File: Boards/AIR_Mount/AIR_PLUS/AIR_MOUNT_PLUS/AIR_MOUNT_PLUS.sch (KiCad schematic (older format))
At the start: 10 parts, among them J1 UF_4_VT, J2 MicroFit_VT_4, J4 redcude_7461166, J5 redcude_7461166, K1 LI12-1A85(NO), U1 MicroFit_VT_6

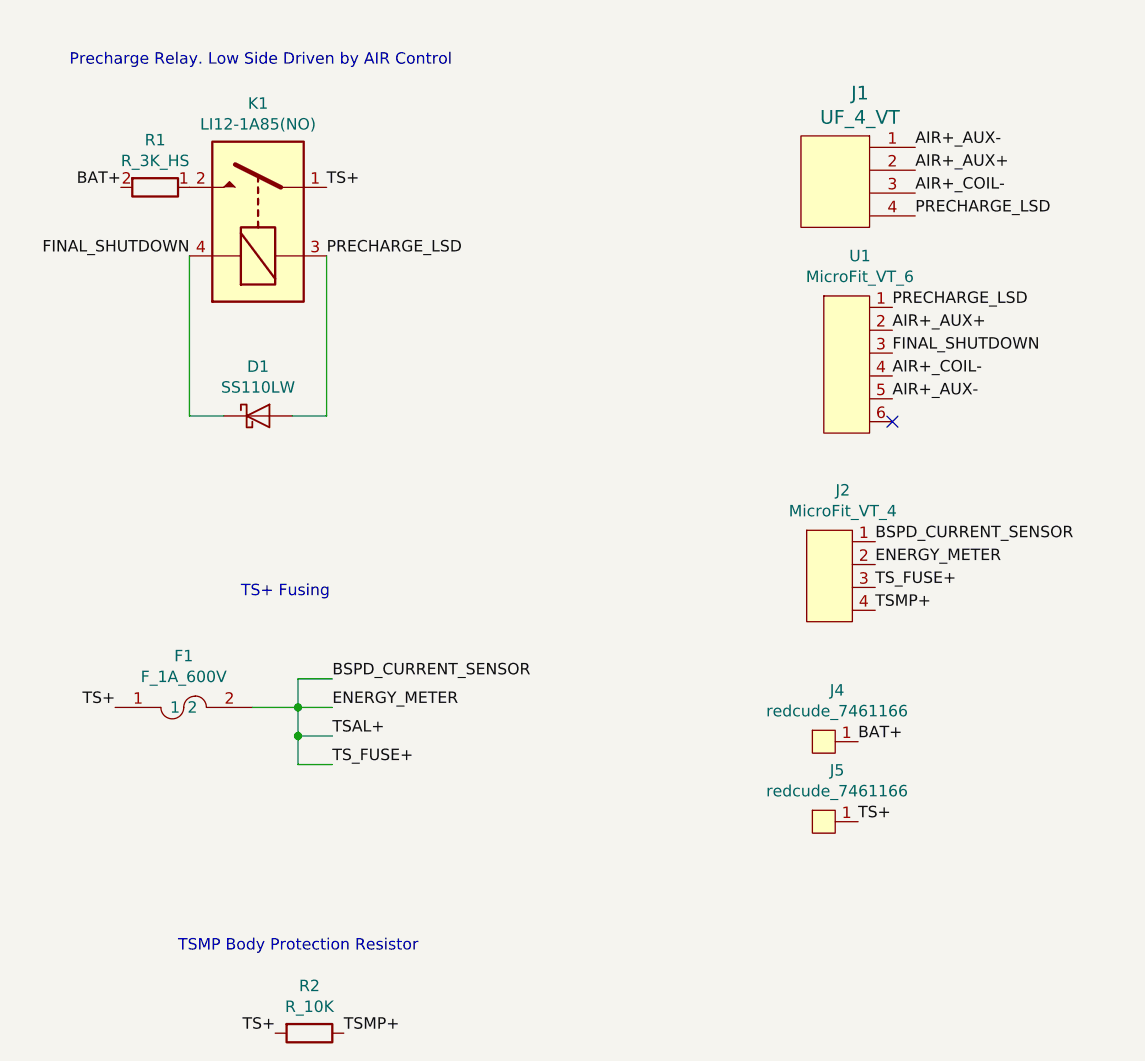
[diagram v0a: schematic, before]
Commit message: Updating AIR Mount Boards
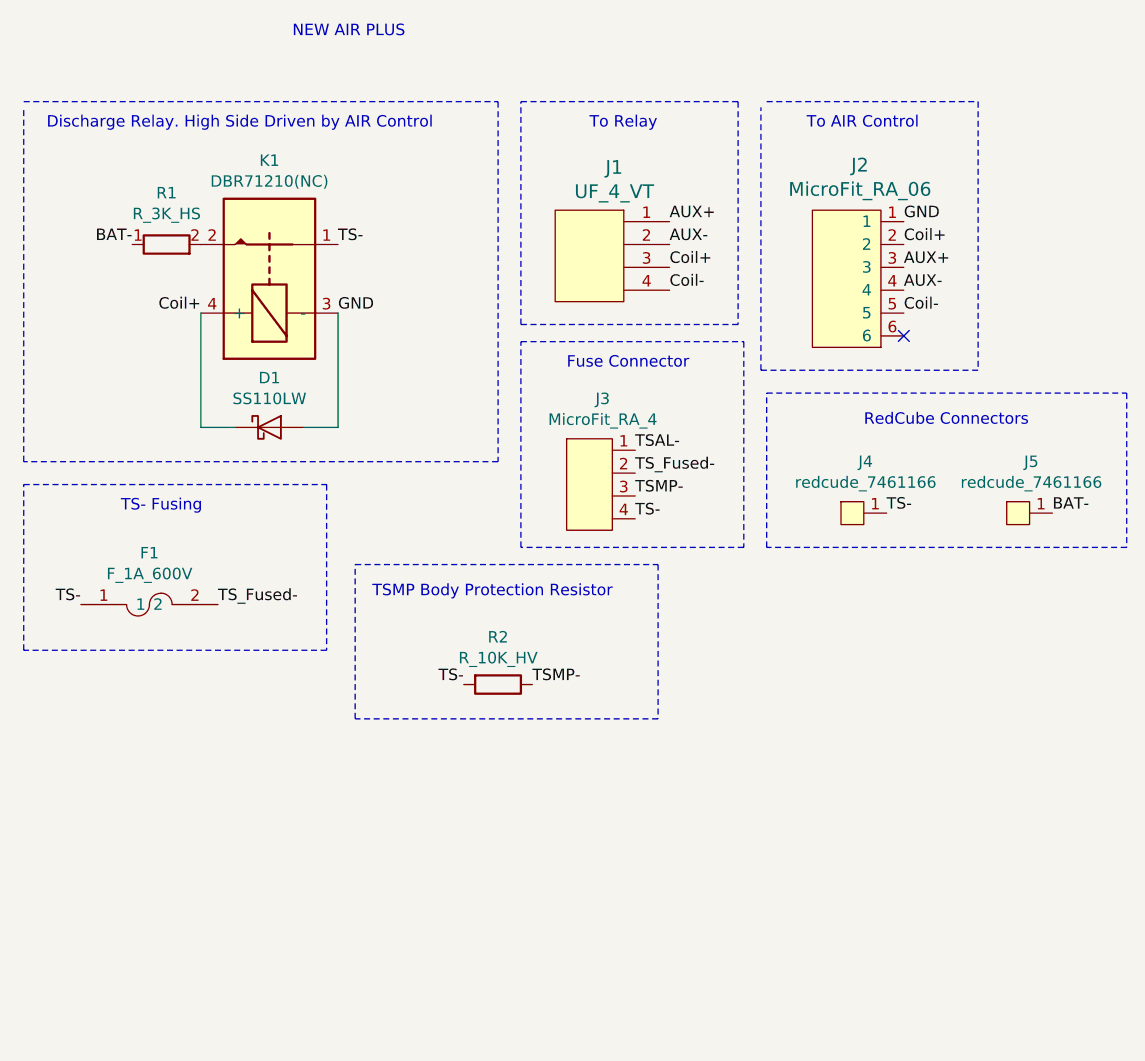
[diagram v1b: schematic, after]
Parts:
- removed D1: SS110LW, footprints:D_SOD-123W_OEM, symbol AIR_MOUNT_PLUS-rescue:SS110LW-formula
- removed J1: UF_4_VT, footprints:Ultrafit_4, symbol AIR_MOUNT_PLUS-rescue:UF_4_VT-footprints
- removed J2: MicroFit_VT_4, footprints:MicroFit_VT_4, symbol AIR_MOUNT_PLUS-rescue:MicroFit_VT_4-footprints
- removed J4, J5: redcude_7461166, footprints:redcube_7461166, symbol AIR_MOUNT_PLUS-rescue:redcude_7461166-footprints
- removed K1: LI12-1A85(NO), footprints:Meder-LI12, symbol AIR_MOUNT_PLUS-rescue:LI12-1A85(NO)-formula
- removed R1: R_3K_HS, footprints:R_3k_HS_TO247, symbol AIR_MOUNT_PLUS-rescue:R_3K_HS-formula
- removed R2: R_10K, footprints:R_TSMP_SMD_5329, symbol Device:R
- removed U1: MicroFit_VT_6, footprints:MicroFit_VT_6, symbol AIR_MOUNT_PLUS-rescue:MicroFit_VT_6-footprints
- added D1: SS110LW, footprints:D_SOD-123W_OEM, symbol Formula:SS110LW
- added J1: UF_4_VT, footprints:Ultrafit_4, symbol Formula:UF_4_VT
- added J2: MicroFit_RA_06, footprints:MicroFit_RA_06, symbol Formula:MicroFit_RA_06
- added J3: MicroFit_RA_4, footprints:MicroFit_RA_4, symbol Formula:MicroFit_RA_4
- added J4, J5: redcude_7461166, footprints:redcube_7461166, symbol Formula:redcude_7461166
- added K1: DBR71210(NC), footprints:D-Series_Cynergy_Relay, symbol Formula:DBR71210(NC)
- added R1: R_3K_HS, footprints:R_3k_HS_TO247, symbol Formula:R_3K_HS
- added R2: R_10K_HV, footprints:R_TSMP_SMD_5329, symbol Formula:R_10K_HV
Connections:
- net BSPD_CURRENT_SENSOR renamed TS_Fused-
- net TS_Fused-: now also J3.2
- net TS+ renamed TS-
- net TS-: now also J3.4, J4.1, K1.1, R2.2
- new net: K1.2, R1.2
- new net AUX+: J1.1, J2.3
- new net AUX-: J1.2, J2.4
- new net BAT-: J5.1, R1.1
- new net Coil+: D1.1 (K), J1.3, J2.2, K1.4 (+)
- new net Coil-: J1.4, J2.5
- new net GND: D1.2 (A), J2.1, K1.3 (-)
- new net TSAL-: J3.1
- new net TSMP-: J3.3, R2.1
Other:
- note added: "Discharge Relay. High Side Driven by AIR Control"
- note added: "Fuse Connector"
- note added: "NEW AIR PLUS\n"
- note added: "RedCube Connectors"
- note added: "TS- Fusing"
- note added: "To AIR Control\n"
- note added: "To Relay\n"
- note removed: "Precharge Relay. Low Side Driven by AIR Control\n"
- note removed: "TS+ Fusing"
